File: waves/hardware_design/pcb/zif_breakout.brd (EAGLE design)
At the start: 23.9 x 19.3 mm, 6 parts, among them J8 F31L-1A7H1-11030

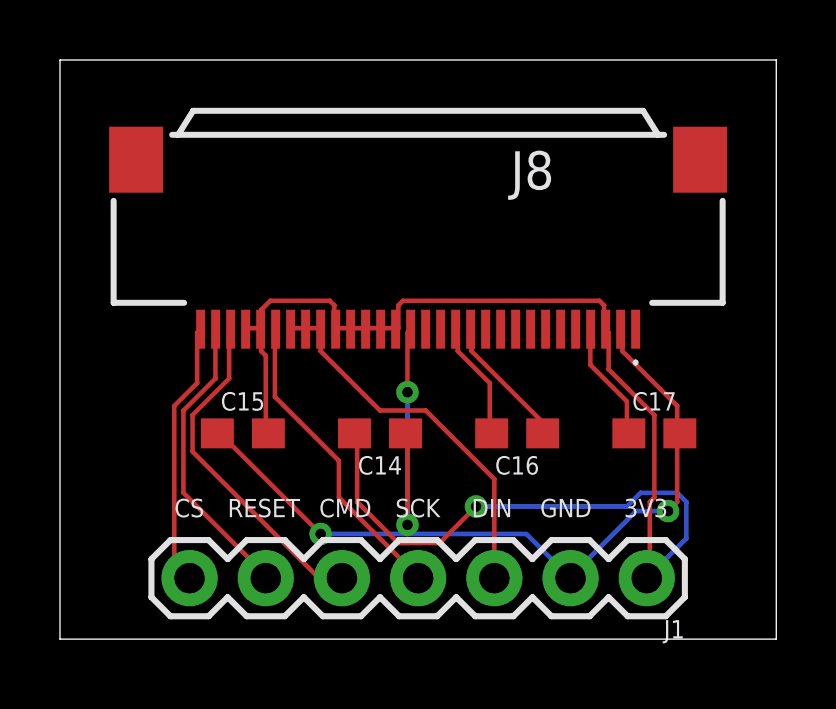
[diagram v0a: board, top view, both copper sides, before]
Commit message: trying to get LCD to respond
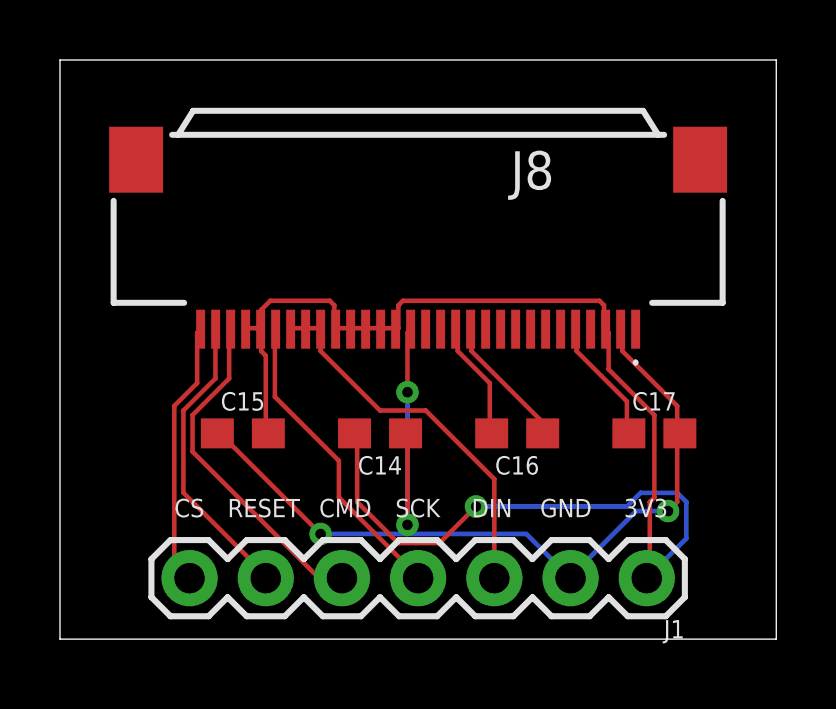
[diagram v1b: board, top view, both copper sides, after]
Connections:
- net N$3: now also J8.5; no longer J8.4
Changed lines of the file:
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@@
 </signal>
 <signal name="N$3">
-<contactref element="J8" pad="4"/>
 <contactref element="C17" pad="1"/>
+<contactref element="J8" pad="5"/>
 <wire x1="18.8976" y1="7.9248" x2="18.8976" y2="6.858" width="0.1524" layer="1"/>
-<wire x1="17.6784" y1="9.144" x2="18.8976" y2="7.9248" width="0.1524" layer="1"/>
-<wire x1="17.6784" y1="10.2108" x2="17.6784" y2="9.144" width="0.1524" layer="1"/>
+<wire x1="17.2212" y1="9.6012" x2="18.8976" y2="7.9248" width="0.1524" layer="1"/>
+<wire x1="17.2212" y1="10.2108" x2="17.2212" y2="9.6012" width="0.1524" layer="1"/>
 <wire x1="18.8976" y1="6.858" x2="18.962" y2="6.858" width="0.1524" layer="1"/>
-<wire x1="17.6784" y1="10.2108" x2="17.688" y2="10.33" width="0.1524" layer="1"/>
+<wire x1="17.2212" y1="10.2108" x2="17.188" y2="10.33" width="0.1524" layer="1"/>
 </signal>
 <signal name="N$12">
